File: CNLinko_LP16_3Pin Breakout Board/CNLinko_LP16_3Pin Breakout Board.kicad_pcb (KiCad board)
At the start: 2 copper layers, 31.8 x 25.4 mm, 2 parts, among them J1 Conn_01x03

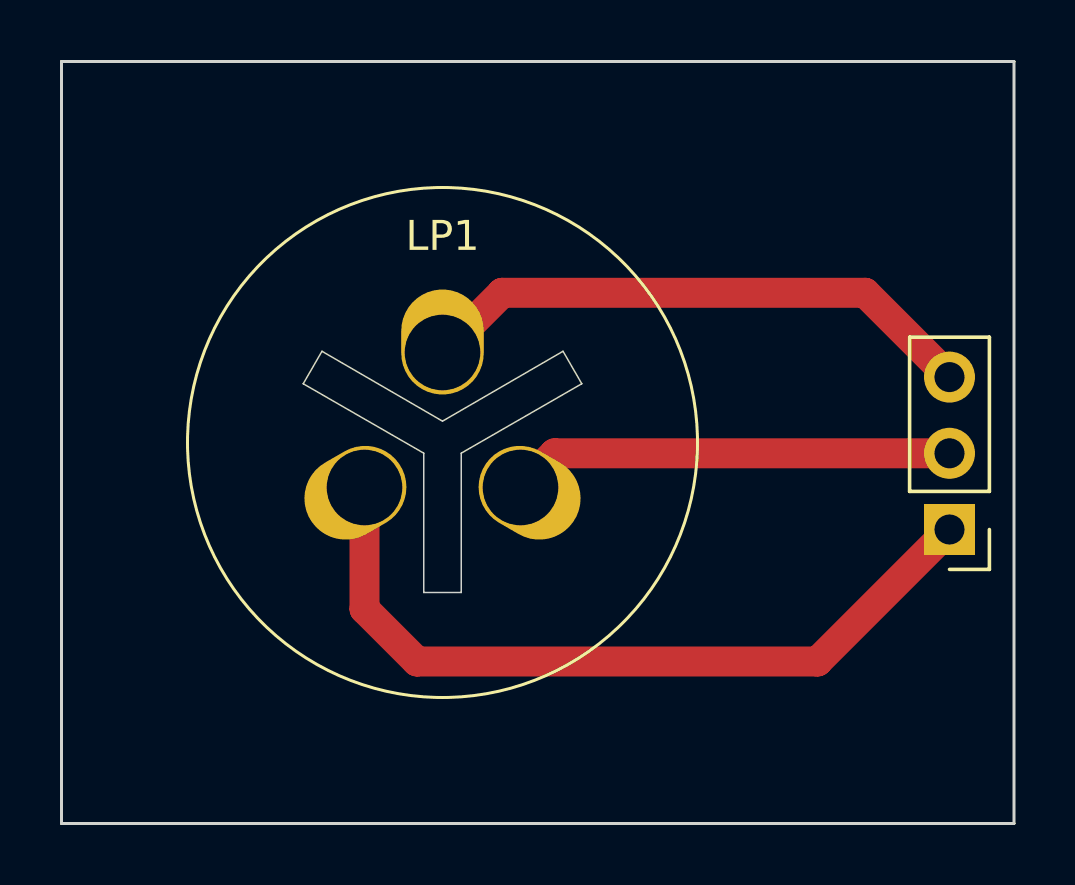
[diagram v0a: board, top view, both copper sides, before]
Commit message: AAAAAAAAAA
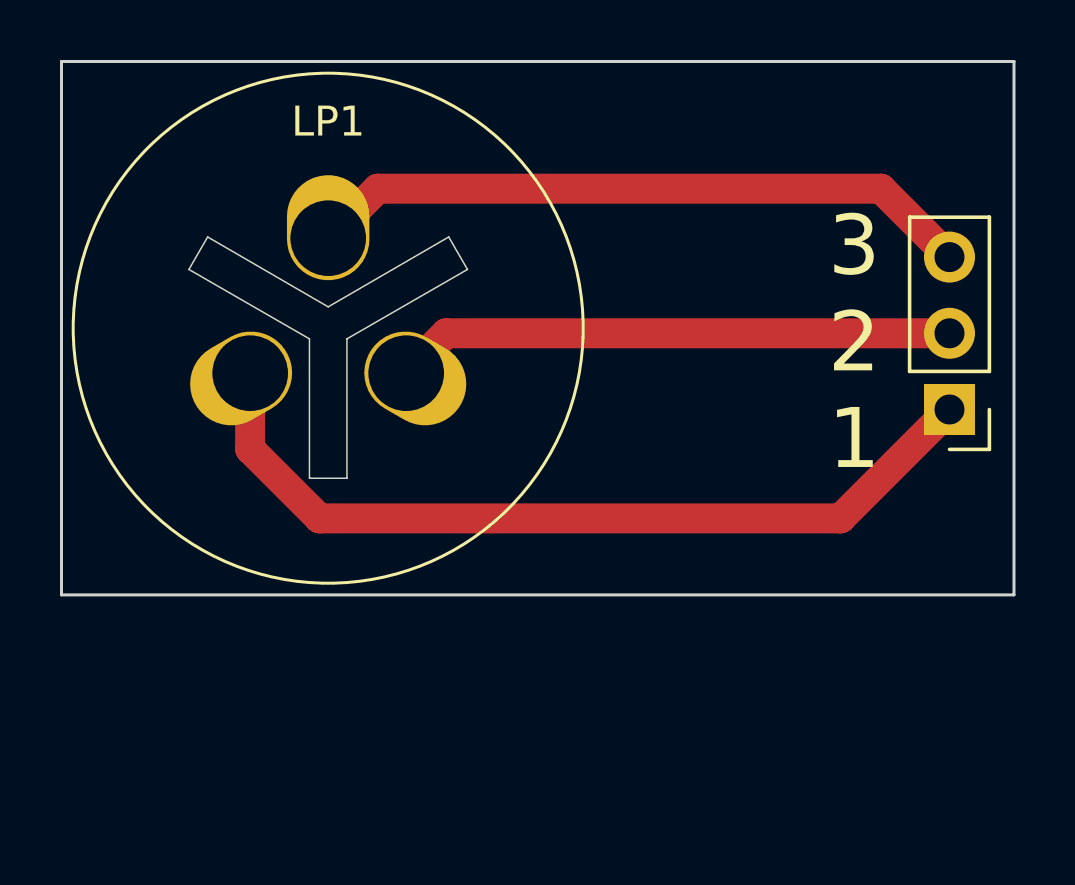
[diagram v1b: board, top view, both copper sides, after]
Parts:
- added G***: LOGO, LOGO:RP_Logo, B.Cu at (43.9, 30.8)
- moved LP1 5.39 mm to (34.3, 34.3)
- moved J1 4.00 mm to (55.0, 37.0)
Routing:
- net Pin 2: track 14.8 -> 18.7 mm
- net Pin 3: track 18.9 -> 22.3 mm
- net Pin 1: track 26.1 -> 28.3 mm
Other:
- board size 31.8 x 25.4 mm -> 31.8 x 17.8 mm
- board text added: "3 2 1"
- board text added: "LP16-3Pin"
